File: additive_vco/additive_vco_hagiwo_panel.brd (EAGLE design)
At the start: 30 x 115 mm, 0 parts

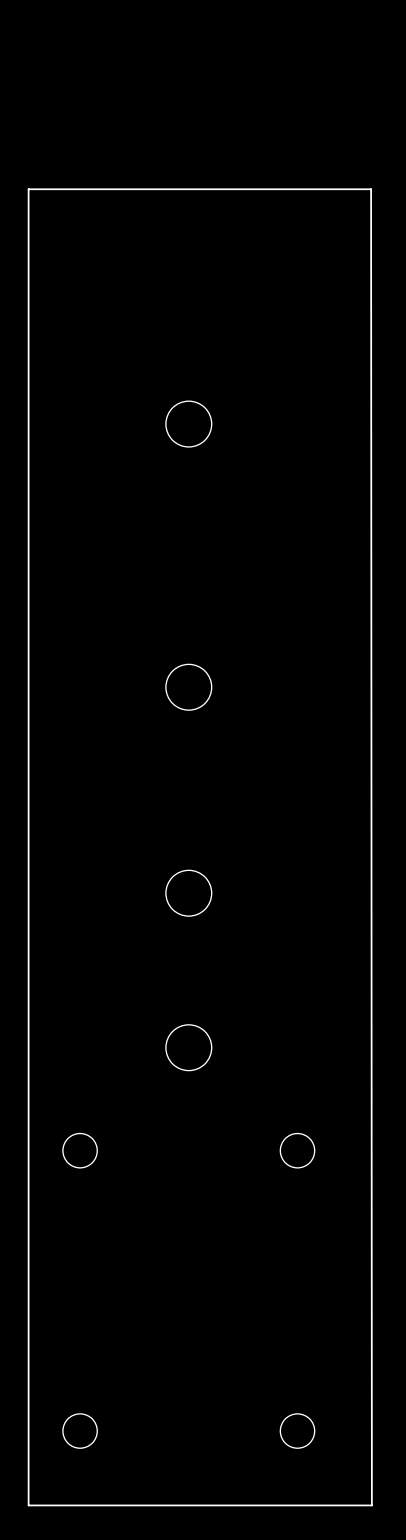
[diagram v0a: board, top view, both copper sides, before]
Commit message: better front panel
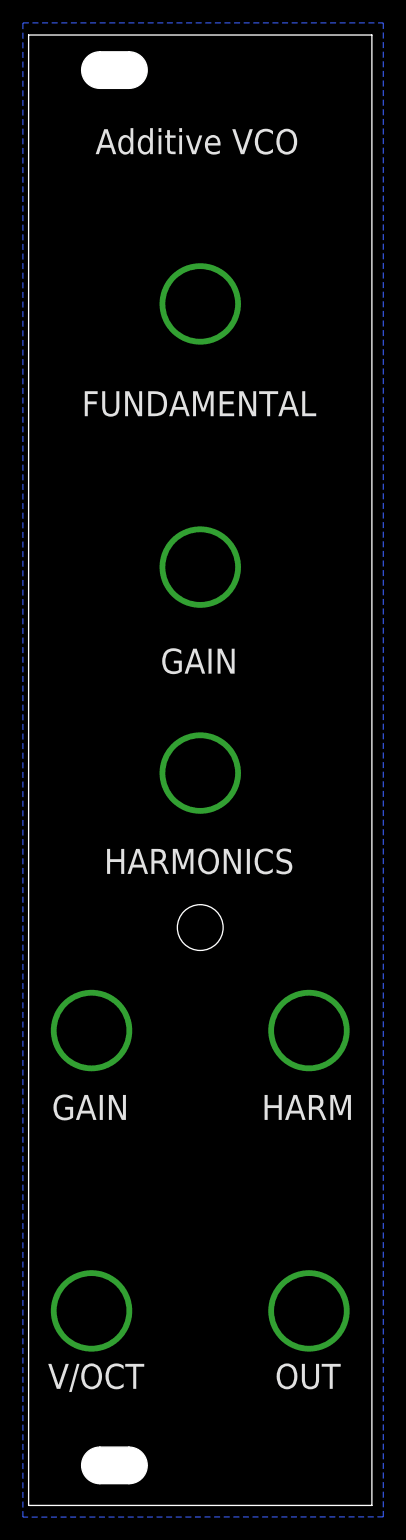
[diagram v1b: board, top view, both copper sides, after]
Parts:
- added U$1, U$2: (no value), MusicThingModular:SLOT_HOLE
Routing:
- added copper zone on layer 16, net GND
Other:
- board size 30 x 115 mm -> 30 x 128.5 mm
- board text added: "Additive VCO"
- board text added: "FUNDAMENTAL"
- board text added: "GAIN"
- board text added: "HARM"
- board text added: "HARMONICS"
- board text added: "OUT"
- board text added: "V/OCT"

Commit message: submit to pcb fab
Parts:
- added E$1: (no value), todstuff:ADDITIVE_VCO_PANEL1
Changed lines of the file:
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@@
 <layer number="56" name="wert" color="7" fill="1" visible="no" active="no"/>
 <layer number="57" name="tCAD" color="7" fill="1" visible="no" active="no"/>
+<layer number="59" name="tCarbon" color="7" fill="1" visible="no" active="no"/>
+<layer number="60" name="bCarbon" color="7" fill="1" visible="no" active="no"/>
+<layer number="88" name="SimResults" color="9" fill="1" visible="no" active="no"/>
+<layer number="89" name="SimProbes" color="9" fill="1" visible="no" active="no"/>
 <layer number="90" name="Modules" color="5" fill="1" visible="no" active="no"/>
 <layer number="91" name="Nets" color="2" fill="1" visible="no" active="no"/>
@@
 <layer number="111" name="111" color="7" fill="1" visible="no" active="no"/>
 <layer number="112" name="tSilk" color="7" fill="1" visible="no" active="no"/>
+<layer number="113" name="IDFDebug" color="4" fill="1" visible="no" active="no"/>
+<layer number="114" name="Badge_Outline" color="7" fill="1" visible="no" active="yes"/>
+<layer number="115" name="ReferenceISLANDS" color="7" fill="1" visible="no" active="yes"/>
 <layer number="116" name="Patch_BOT" color="9" fill="4" visible="yes" active="yes"/>
 <layer number="118" name="Rect_Pads" color="7" fill="1" visible="no" active="no"/>
@@
 <layer number="127" name="_tValues" color="7" fill="1" visible="no" active="no"/>
 <layer number="128" name="_bValues" color="7" fill="1" visible="no" active="no"/>
+<layer number="129" name="Mask" color="7" fill="1" visible="no" active="no"/>
 <layer number="131" name="prix" color="7" fill="1" visible="no" active="yes"/>
 <layer number="132" name="test" color="7" fill="1" visible="no" active="yes"/>
@@
 <layer number="223" name="223bmp" color="24" fill="1" visible="no" active="no"/>
 <layer number="224" name="224bmp" color="25" fill="1" visible="no" active="no"/>
+<layer number="225" name="225bmp" color="7" fill="1" visible="no" active="no"/>
+<layer number="226" name="226bmp" color="7" fill="1" visible="no" active="no"/>
+<layer number="227" name="227bmp" color="7" fill="1" visible="no" active="no"/>
+<layer number="228" name="228bmp" color="7" fill="1" visible="no" active="no"/>
+<layer number="229" name="229bmp" color="7" fill="1" visible="no" active="no"/>
+<layer number="230" name="230bmp" color="7" fill="1" visible="no" active="no"/>
+<layer number="231" name="231bmp" color="7" fill="1" visible="no" active="no"/>
+<layer number="232" name="Eagle3D_PG2" color="7" fill="1" visible="no" active="no"/>
+<layer number="233" name="Eagle3D_PG3" color="7" fill="1" visible="no" active="no"/>
 <layer number="248" name="Housing" color="7" fill="1" visible="no" active="no"/>
 <layer number="249" name="Edge" color="7" fill="1" visible="no" active="no"/>
@@
 <layer number="251" name="SMDround" color="12" fill="11" visible="no" active="no"/>
 <layer number="254" name="cooling" color="7" fill="1" visible="no" active="yes"/>
+<layer number="255" name="routoute" color="7" fill="1" visible="no" active="no"/>
 </layers>
 <board>
@@
 <element name="U$1" library="MusicThingModular" package="SLOT_HOLE" value="" x="7.5" y="3.5" smashed="yes" rot="R180"/>
 <element name="U$2" library="MusicThingModular" package="SLOT_HOLE" value="" x="7.5" y="125.4365" smashed="yes" rot="R180"/>
+<element name="E$1" library="todstuff" library_urn="urn:adsk.eagle:library:1731349" package="ADDITIVE_VCO_PANEL1" value="" x="0" y="0" smashed="yes"/>
 </elements>
 <signals>
@@
 </board>
 </drawing>
+<compatibility>
+<note version="8.2" severity="warning">
+Since Version 8.2, EAGLE supports online libraries. The ids
+of those online libraries will not be understood (or retained)
+with this version.
+</note>
+</compatibility>
 </eagle>
